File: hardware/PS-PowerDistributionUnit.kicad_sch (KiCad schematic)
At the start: 5 parts, among them J1 XT-30, J2 Molex_NanoFit_1x2, J3 Molex_NanoFit_1x2

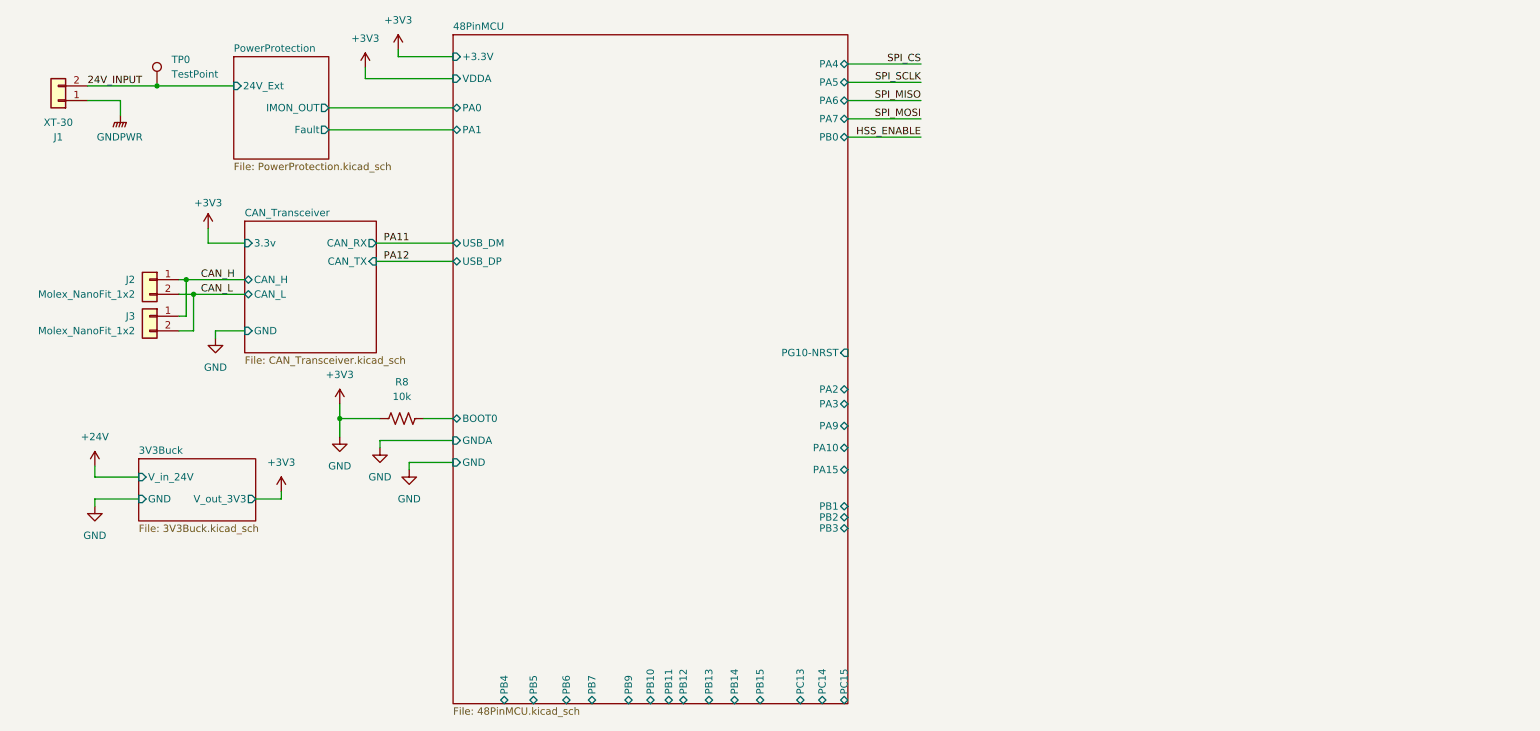
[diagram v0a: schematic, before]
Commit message: progress before drive back to austin
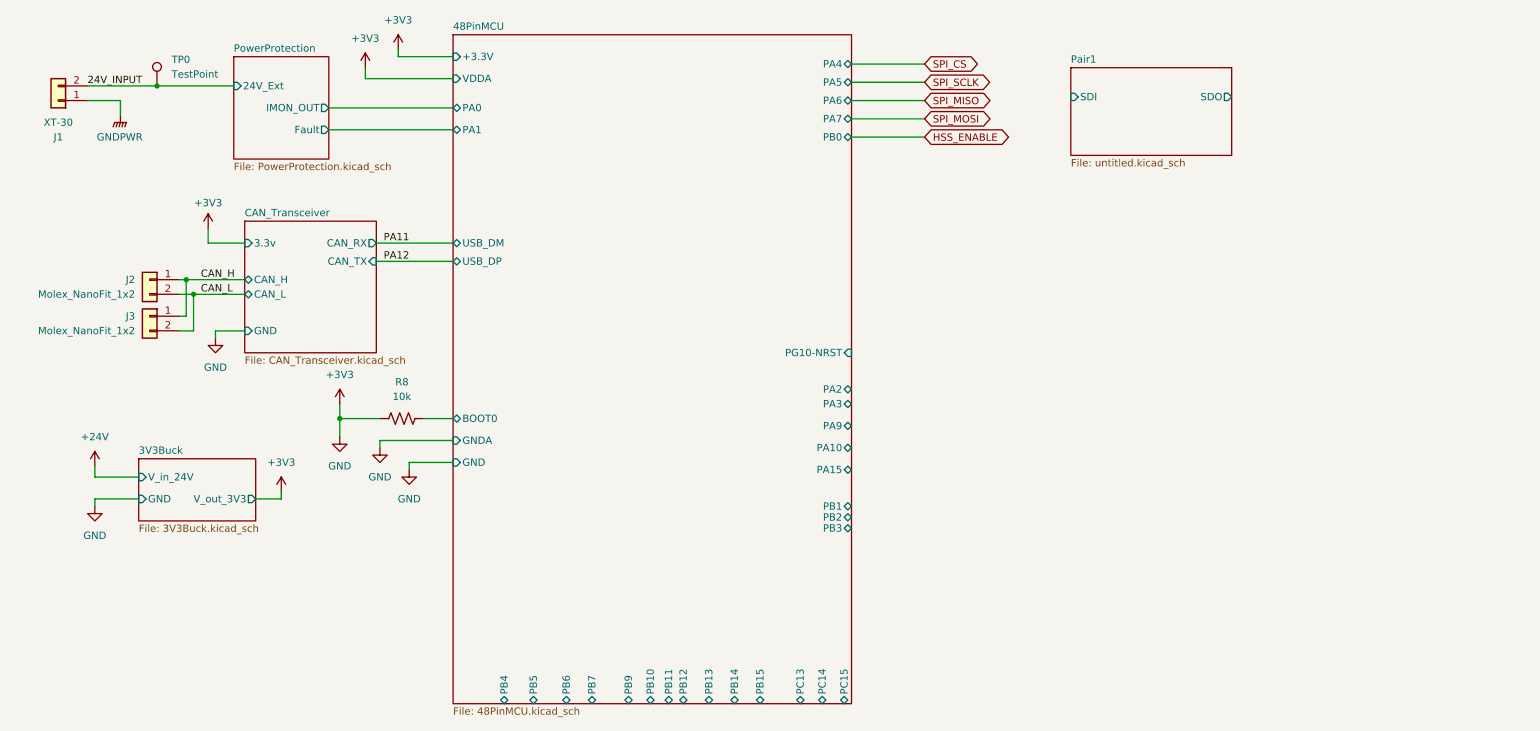
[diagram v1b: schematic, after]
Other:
- added sheet Pair1 (untitled.kicad_sch)
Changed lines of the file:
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@@
+	(wire
+		(pts
+			(xy 156.21 26.67) (xy 168.91 26.67)
+		)
+		(stroke
+			(width 0)
+			(type default)
+		)
+	)
 	(wire
 		(pts
@@
 	(wire
 		(pts
-			(xy 155.575 29.845) (xy 168.275 29.845)
-		)
-		(stroke
-			(width 0)
-			(type default)
-		)
-	)
-	(wire
-		(pts
-			(xy 155.575 36.195) (xy 168.275 36.195)
+			(xy 156.21 29.845) (xy 168.91 29.845)
 		)
 		(stroke
@@
 	(wire
 		(pts
-			(xy 155.575 33.02) (xy 168.275 33.02)
+			(xy 156.21 33.02) (xy 168.91 33.02)
 		)
 		(stroke
@@
 	(wire
 		(pts
+			(xy 156.21 36.195) (xy 168.91 36.195)
+		)
+		(stroke
+			(width 0)
+			(type default)
+		)
+	)
+	(wire
+		(pts
 			(xy 74.295 88.9) (xy 86.995 88.9)
 		)
@@
 	(wire
 		(pts
-			(xy 155.575 26.67) (xy 168.275 26.67)
-		)
-		(stroke
-			(width 0)
-			(type default)
-		)
-	)
-	(wire
-		(pts
 			(xy 45.72 69.85) (xy 50.8 69.85)
 		)
@@
 	(wire
 		(pts
-			(xy 155.575 23.495) (xy 168.275 23.495)
+			(xy 156.21 23.495) (xy 168.91 23.495)
 		)
 		(stroke
@@
 			(width 0)
 			(type default)
-		)
-	)
-	(label "HSS_ENABLE"
-		(at 168.275 36.195 180)
-		(effects
-			(font
-				(size 1.27 1.27)
-			)
-			(justify right bottom)
-		)
-	)
-	(label "SPI_CS"
-		(at 168.275 23.495 180)
-		(effects
-			(font
-				(size 1.27 1.27)
-			)
-			(justify right bottom)
-		)
-	)
-	(label "SPI_MOSI"
-		(at 168.275 33.02 180)
-		(effects
-			(font
-				(size 1.27 1.27)
-			)
-			(justify right bottom)
 		)
 	)
@@
 		)
 	)
-	(label "SPI_SCLK"
-		(at 168.275 26.67 180)
+	(global_label "SPI_CS"
+		(shape bidirectional)
+		(at 168.91 23.495 0)
+		(fields_autoplaced yes)
 		(effects
 			(font
 				(size 1.27 1.27)
 			)
-			(justify right bottom)
-		)
-	)
-	(label "SPI_MISO"
-		(at 168.275 29.845 180)
+			(justify left)
+		)
+		(property "Intersheetrefs" "${INTERSHEET_REFS}"
+			(at 179.5379 23.495 0)
+			(effects
+				(font
+					(size 1.27 1.27)
+				)
+				(justify left)
+				(hide yes)
+			)
+		)
+	)
+	(global_label "SPI_SCLK"
+		(shape bidirectional)
+		(at 168.91 26.67 0)
+		(fields_autoplaced yes)
 		(effects
 			(font
 				(size 1.27 1.27)
 			)
-			(justify right bottom)
+			(justify left)
+		)
+		(property "Intersheetrefs" "${INTERSHEET_REFS}"
+			(at 181.836 26.67 0)
+			(effects
+				(font
+					(size 1.27 1.27)
+				)
+				(justify left)
+				(hide yes)
+			)
+		)
+	)
+	(global_label "SPI_MOSI"
+		(shape bidirectional)
+		(at 168.91 33.02 0)
+		(fields_autoplaced yes)
+		(effects
+			(font
+				(size 1.27 1.27)
+			)
+			(justify left)
+		)
+		(property "Intersheetrefs" "${INTERSHEET_REFS}"
+			(at 181.6546 33.02 0)
+			(effects
+				(font
+					(size 1.27 1.27)
+				)
+				(justify left)
+				(hide yes)
+			)
+		)
+	)
+	(global_label "SPI_MISO"
+		(shape bidirectional)
+		(at 168.91 29.845 0)
+		(fields_autoplaced yes)
+		(effects
+			(font
+				(size 1.27 1.27)
+			)
+			(justify left)
+		)
+		(property "Intersheetrefs" "${INTERSHEET_REFS}"
+			(at 181.6546 29.845 0)
+			(effects
+				(font
+					(size 1.27 1.27)
+				)
+				(justify left)
+				(hide yes)
+			)
+		)
+	)
+	(global_label "HSS_ENABLE"
+		(shape bidirectional)
+		(at 168.91 36.195 0)
+		(fields_autoplaced yes)
+		(effects
+			(font
+				(size 1.27 1.27)
+			)
+			(justify left)
+		)
+		(property "Intersheetrefs" "${INTERSHEET_REFS}"
+			(at 184.7388 36.195 0)
+			(effects
+				(font
+					(size 1.27 1.27)
+				)
+				(justify left)
+				(hide yes)
+			)
 		)
 	)
@@
 	(sheet
 		(at 86.995 18.415)
-		(size 68.58 116.205)
+		(size 69.215 116.205)
 		(exclude_from_sim no)
 		(in_bom yes)
@@
 		)
 		(pin "PA2" bidirectional
-			(at 155.575 80.01 0)
+			(at 156.21 80.01 0)
 			(effects
 				(font
@@
 		)
 		(pin "PA3" bidirectional
-			(at 155.575 82.55 0)
+			(at 156.21 82.55 0)
 			(effects
 				(font
@@
 		)
 		(pin "PA4" bidirectional
-			(at 155.575 23.495 0)
+			(at 156.21 23.495 0)
 			(effects
 				(font
@@
 		)
 		(pin "PA5" bidirectional
-			(at 155.575 26.67 0)
+			(at 156.21 26.67 0)
 			(effects
 				(font
@@
 		)
 		(pin "PA6" bidirectional
-			(at 155.575 29.845 0)
+			(at 156.21 29.845 0)
 			(effects
 				(font
@@
 		)
 		(pin "PA7" bidirectional
-			(at 155.575 33.02 0)
+			(at 156.21 33.02 0)
 			(effects
 				(font
@@
 		)
 		(pin "PA9" bidirectional
-			(at 155.575 86.36 0)
+			(at 156.21 86.36 0)
 			(effects
 				(font
@@
 		)
 		(pin "PA10" bidirectional
-			(at 155.575 90.17 0)
+			(at 156.21 90.17 0)
 			(effects
 				(font
@@
 		)
 		(pin "PA15" bidirectional
-			(at 155.575 93.98 0)
+			(at 156.21 93.98 0)
 			(effects
 				(font
@@
 		)
 		(pin "PB0" bidirectional
-			(at 155.575 36.195 0)
+			(at 156.21 36.195 0)
 			(effects
 				(font
@@
 		)
 		(pin "PB1" bidirectional
-			(at 155.575 100.33 0)
+			(at 156.21 100.33 0)
 			(effects
 				(font
@@
 		)
 		(pin "PB2" bidirectional
-			(at 155.575 102.235 0)
+			(at 156.21 102.235 0)
 			(effects
 				(font
@@
 		)
 		(pin "PB3" bidirectional
-			(at 155.575 104.14 0)
+			(at 156.21 104.14 0)
 			(effects
 				(font
@@
 		)
 		(pin "PG10-NRST" input
-			(at 155.575 73.66 0)
+			(at 156.21 73.66 0)
 			(effects
 				(font
@@
 				)
 			)
+		)
+	)
+	(sheet
+		(at 194.31 24.13)
+		(size 27.94 15.24)
+		(exclude_from_sim no)
+		(in_bom yes)
+		(on_board yes)
+		(dnp no)
+		(fields_autoplaced yes)
+		(stroke
+			(width 0.1524)
+			(type solid)
+		)
+		(fill
+			(color 0 0 0 0.0000)
+		)
+		(property "Sheetname" "Pair1"
+			(at 194.31 23.4184 0)
+			(effects
+				(font
+					(size 1.27 1.27)
+				)
+				(justify left bottom)
+			)
+		)
+		(property "Sheetfile" "untitled.kicad_sch"
+			(at 194.31 39.9546 0)
+			(effects
+				(font
+					(size 1.27 1.27)
+				)
+				(justify left top)
+			)
+		)
+		(pin "SDI" input
+			(at 194.31 29.21 180)
+			(effects
+				(font
+					(size 1.27 1.27)
+				)
+				(justify left)
+			)
+		)
+		(pin "SDO" output
+			(at 222.25 29.21 0)
+			(effects
+				(font
+					(size 1.27 1.27)
+				)
+				(justify right)
+			)
+		)
+		(instances
+			(project "PS-PowerDistributionUnit"
+				(path "/eb16378f-e371-46a9-bfab-b0d9404d0362"
+					(page "6")
+				)
+			)

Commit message: added hss and driving back from houston
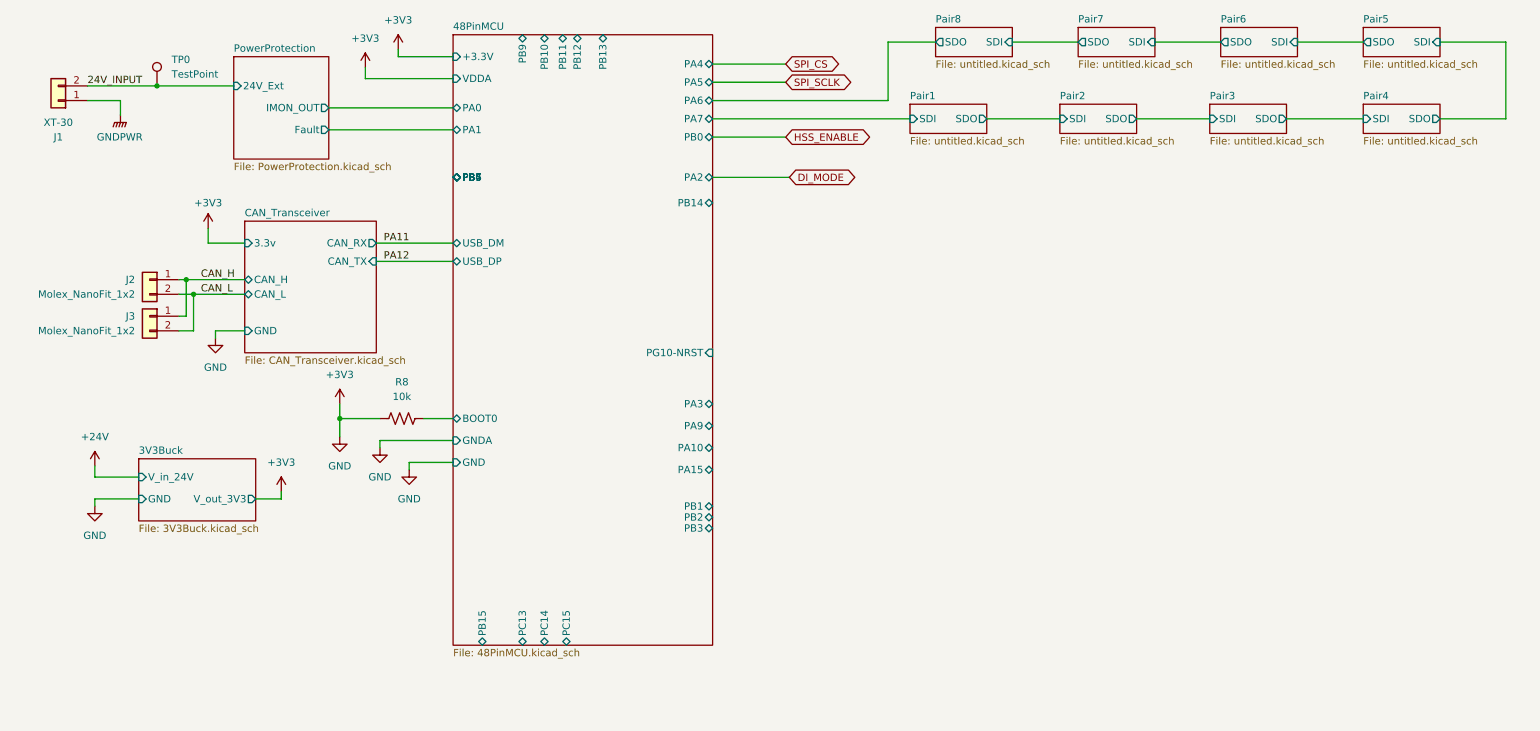
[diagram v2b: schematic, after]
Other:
- added sheet Pair2 (untitled.kicad_sch)
- added sheet Pair3 (untitled.kicad_sch)
- added sheet Pair4 (untitled.kicad_sch)
- added sheet Pair5 (untitled.kicad_sch)
- added sheet Pair6 (untitled.kicad_sch)
- added sheet Pair7 (untitled.kicad_sch)
- added sheet Pair8 (untitled.kicad_sch)
